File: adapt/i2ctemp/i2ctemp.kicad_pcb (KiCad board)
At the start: 2 copper layers, 100 x 80 mm, 9 parts

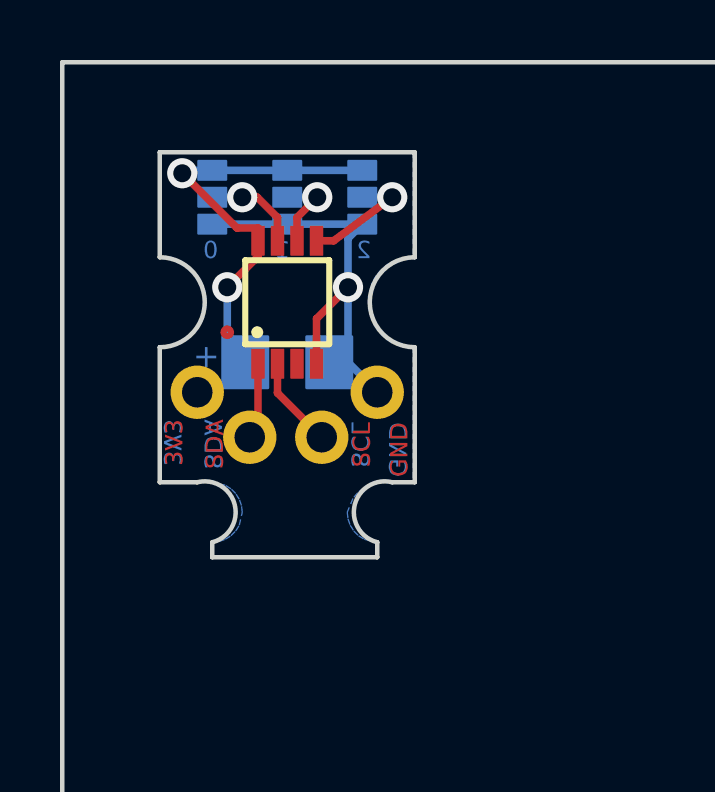
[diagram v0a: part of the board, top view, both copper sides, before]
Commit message: Old check-in: i2ctemp
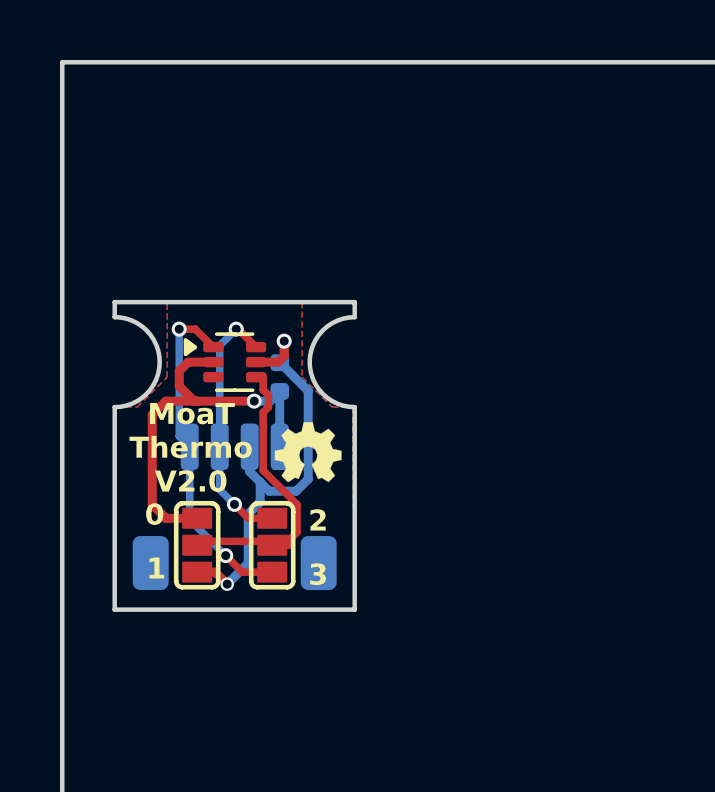
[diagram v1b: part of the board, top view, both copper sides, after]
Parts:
- removed 3V3, GND1, SCK1, SDA1: PINHD-1X1CB, i2ctemp:1X01-CLEANBIG
- removed AJ2: SolderJumper_3_Open, i2ctemp:SJ3_S
- removed TEMP1: MCP9808MSOP, i2ctemp:MSOP8
- added G***: LOGO, localstuff:OSHW Logo 2mm, F.Cu at (106.7, 78.0)
- added J1: Conn_01x04_Pin, Connector_JST:JST_SH_SM04B-SRSS-TB_1x04-1MP_P1.00mm_Horizontal, B.Cu at (104.2, 79.8)
- added U1: TMP102xxDRL, Package_TO_SOT_SMD:SOT-563, F.Cu at (104.2, 75.0)
- AJ0, AJ1: moved to F.Cu
- C1: value CP_1µ_10V_1206 -> C 100nF; footprint i2ctemp:CP1206 -> Capacitor_SMD:C_0402_1005Metric
- moved AJ0 11.6 mm to (103.0, 81.1), turned to -90 degrees
- moved AJ1 11.6 mm to (105.5, 81.1), turned to -90 degrees
- moved C1 0.56 mm to (105.8, 75.5), turned to -90 degrees
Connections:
- AJ1 pad 1: GND -> /SDA
- AJ1 pad 2: /Adr1 -> /Adr0
- AJ1 pad 3: +3V3 -> /SCL
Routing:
- net /SCL: track 3.06 -> 11.4 mm, vias 0 -> 2
- net /Adr0: track 3.23 -> 10.1 mm, vias 1 -> 0
- net /SDA: track 2.56 -> 8.63 mm, vias 0 -> 2
- net /Adr2: track 4.01 -> 0.00 mm, vias 1 -> 0
- net /Adr1: track 2.73 -> 0.00 mm, vias 1 -> 0
- net +3V3: track 16.5 -> 14.8 mm
- net GND: track 14.9 -> 13.7 mm
- added copper zone on F.Cu, net GND
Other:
- outline, holes or cut-outs redrawn
- board text added: "3"
- board text added: "MoaT Thermo V2.0"
- board text removed: "+"
- board text removed: "3V3"
- board text removed: "GND"
- board text removed: "SCL"
- board text removed: "SDA"
